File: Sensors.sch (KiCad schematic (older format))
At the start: 21 parts, among them U1 MCP60x4, U2 HTU21D, U3 PIR

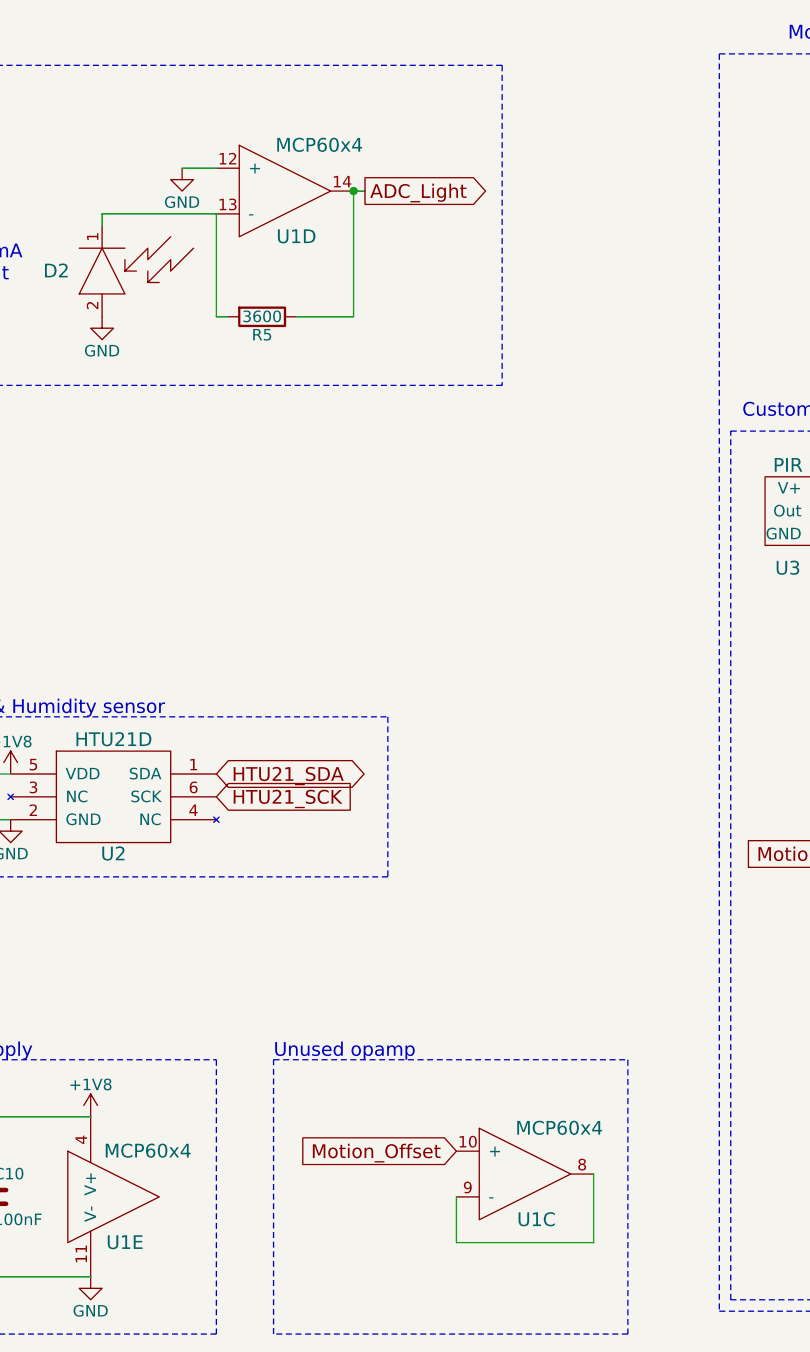
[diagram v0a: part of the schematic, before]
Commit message: Finish routing v4
Signed-off-by: pluyckx <philip.luyckx@gmail.com>
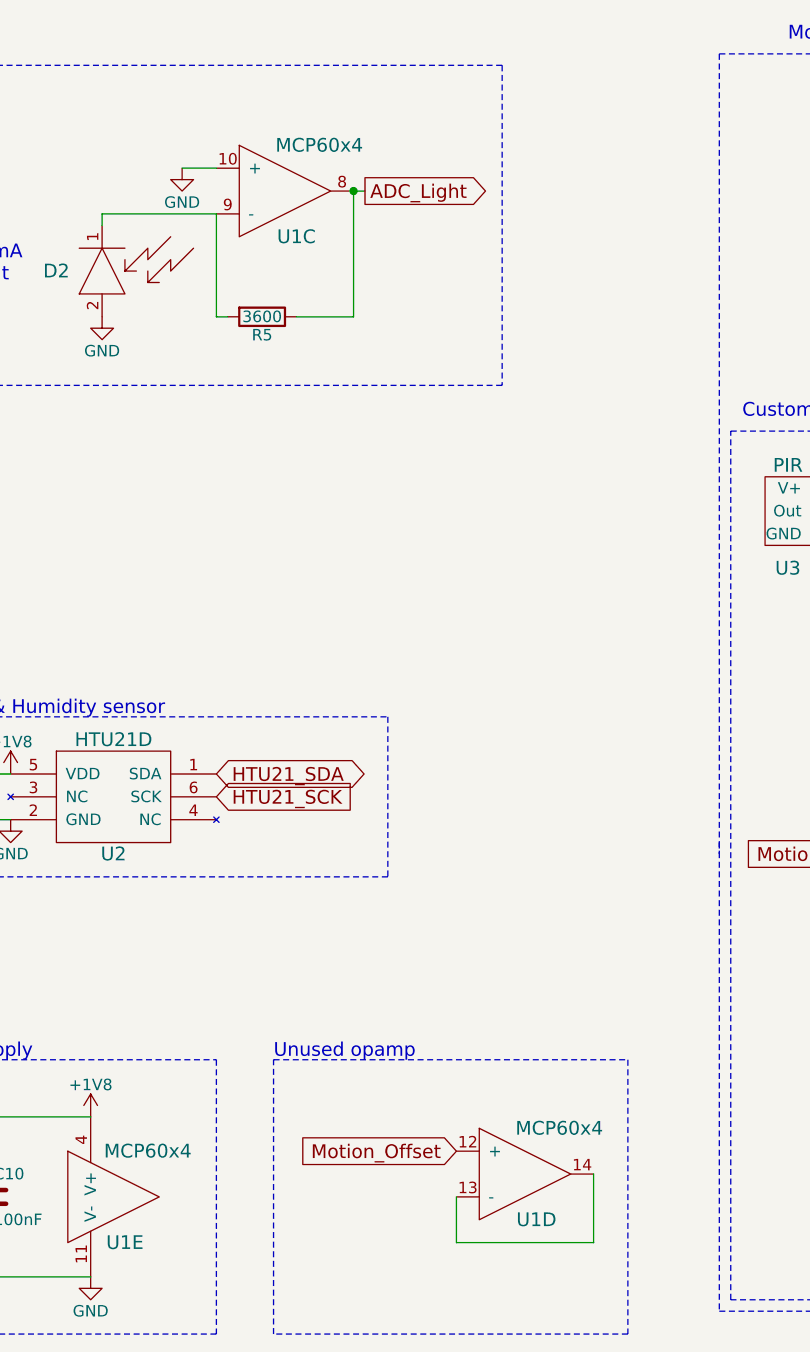
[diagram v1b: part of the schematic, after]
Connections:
- net ADC_Light: now also U1.8; no longer U1.14
- net GND: now also U1.10 (+); no longer U1.12 (+)
- net Motion_Offset: now also U1.12 (+); no longer U1.10 (+)
- net at D2.1, R5.2: now also U1.9 (-); no longer U1.13 (-)
- new net: U1.13 (-), U1.14
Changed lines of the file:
@@
 $Comp
 L MCP60x4 U1
-U 4 1 57538AEE
+U 3 1 57538AEE
 P 2650 1150
 F 0 "U1" H 2750 750 60  0000 C CNN
@@
 F 2 "CustomSmd:SOIC-14" H 2650 1150 60  0001 C CNN
 F 3 "" H 2650 1150 60  0000 C CNN
-	4    2650 1150
+	3    2650 1150
 	1    0    0    -1
 $EndComp
@@
 $Comp
 L MCP60x4 U1
-U 3 1 57538FA3
+U 4 1 57538FA3
 P 3700 5450
 F 0 "U1" H 3800 5050 60  0000 C CNN
@@
 F 2 "CustomSmd:SOIC-14" H 3700 5450 60  0001 C CNN
 F 3 "" H 3700 5450 60  0000 C CNN
-	3    3700 5450
+	4    3700 5450
 	1    0    0    -1
 $EndComp

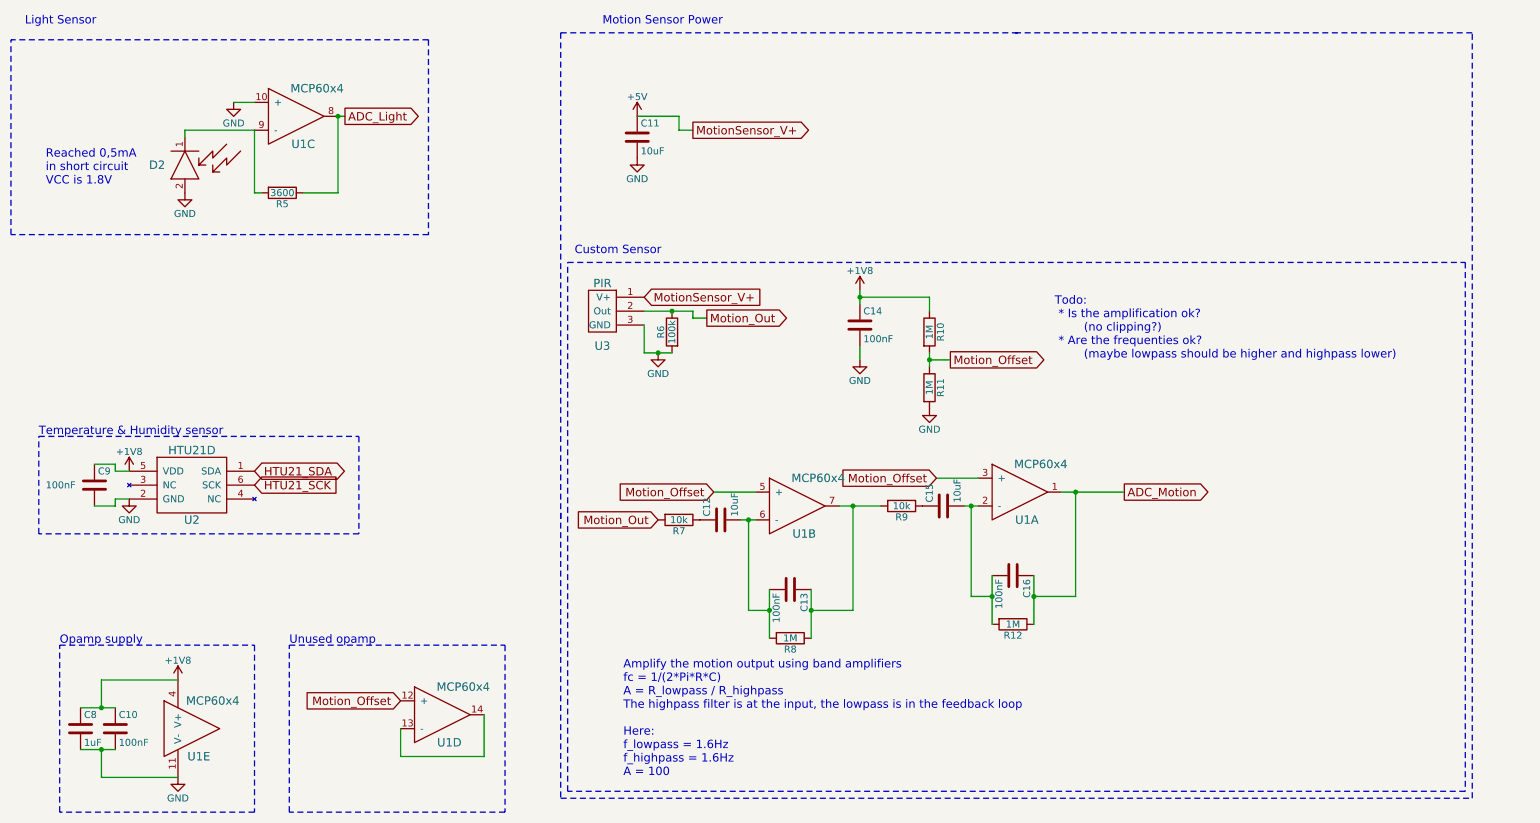
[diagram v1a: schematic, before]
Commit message: Update some routing
Signed-off-by: pluyckx <philip.luyckx@gmail.com>
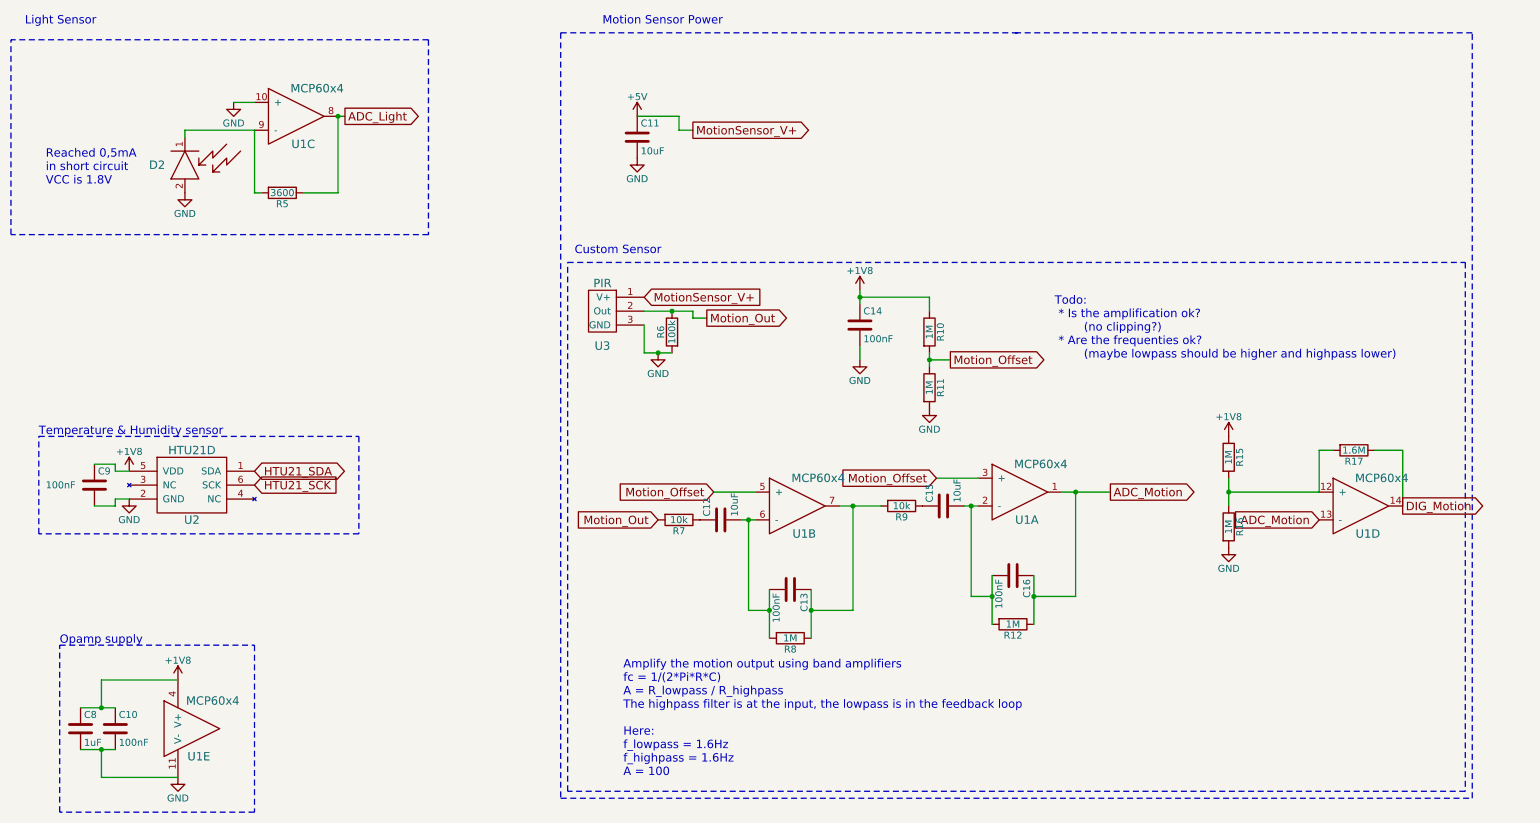
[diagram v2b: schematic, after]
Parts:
- added R15, R16: 1M, Resistors_SMD:R_0603, symbol R
- added R17: 1.6M, Resistors_SMD:R_0603, symbol R
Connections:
- net +1V8: now also R15.1
- net ADC_Motion: now also U1.13 (-)
- net GND: now also R16.2
- net Motion_Offset: no longer U1.12 (+)
- net DIG_Motion: now reaches U1.14
- net DIG_Motion: now also R17.1; no longer U1.13 (-)
- new net: R15.2, R16.1, R17.2, U1.12 (+)
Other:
- note removed: "Unused opamp"
- moved on the sheet: U1D
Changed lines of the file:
@@
 Wire Wire Line
 	8300 4800 8300 4050
-Wire Wire Line
-	8200 4050 8650 4050
 Connection ~ 8000 4800
 Wire Wire Line
@@
 Connection ~ 6700 4150
 Connection ~ 8300 4050
-Text GLabel 8650 4050 2    60   Output ~ 0
+Text GLabel 8550 4050 2    60   Output ~ 0
 ADC_Motion
 Text Notes 5050 6100 0    60   ~ 0
@@
 Text Notes 850  3650 0    60   ~ 0
 Temperature & Humidity sensor
-Wire Wire Line
-	3450 5750 3450 5950
-Wire Wire Line
-	3450 5950 4050 5950
 $Comp
 L MCP60x4 U1
@@
 L MCP60x4 U1
 U 4 1 57538FA3
-P 3700 5450
-F 0 "U1" H 3800 5050 60  0000 C CNN
-F 1 "MCP60x4" H 3900 5450 60  0000 C CNN
-F 2 "CustomSmd:SOIC-14" H 3700 5450 60  0001 C CNN
-F 3 "" H 3700 5450 60  0000 C CNN
-	4    3700 5450
+P 10300 3950
+F 0 "U1" H 10400 3550 60  0000 C CNN
+F 1 "MCP60x4" H 10500 3950 60  0000 C CNN
+F 2 "CustomSmd:SOIC-14" H 10300 3950 60  0001 C CNN
+F 3 "" H 10300 3950 60  0000 C CNN
+	4    10300 3950
 	1    0    0    -1
 $EndComp
@@
 Wire Wire Line
 	1300 5400 1850 5400
-Wire Wire Line
-	4050 5950 4050 5650
-Text GLabel 3450 5550 0    60   Input ~ 0
-Motion_Offset
 Wire Notes Line
 	1000 5150 2400 5150
@@
 Wire Notes Line
 	1000 6350 1000 5150
-Wire Notes Line
-	2650 5150 4200 5150
-Wire Notes Line
-	4200 5150 4200 6350
-Wire Notes Line
-	4200 6350 2650 6350
-Wire Notes Line
-	2650 6350 2650 5150
 Text Notes 1000 5150 0    60   ~ 0
 Opamp supply
-Text Notes 2650 5150 0    60   ~ 0
-Unused opamp
 Wire Wire Line
 	7250 2650 7250 2750
@@
 	1    0    0    -1
 $EndComp
+Text GLabel 10050 4250 0    60   Input ~ 0
+ADC_Motion
+$Comp
+L R R15
+U 1 1 57802832
+P 9400 3800
+F 0 "R15" V 9480 3800 50  0000 C CNN
+F 1 "1M" V 9400 3800 50  0000 C CNN
+F 2 "Resistors_SMD:R_0603" V 9330 3800 50  0001 C CNN
+F 3 "" H 9400 3800 50  0000 C CNN
+	1    9400 3800
+	1    0    0    -1
+$EndComp
+$Comp
+L R R16
+U 1 1 578028BF
+P 9400 4300
+F 0 "R16" V 9480 4300 50  0000 C CNN
+F 1 "1M" V 9400 4300 50  0000 C CNN
+F 2 "Resistors_SMD:R_0603" V 9330 4300 50  0001 C CNN
+F 3 "" H 9400 4300 50  0000 C CNN
+	1    9400 4300
+	1    0    0    -1
+$EndComp
+$Comp
+L +1V8 #PWR031
+U 1 1 5780291A
+P 9400 3650
+F 0 "#PWR031" H 9400 3500 50  0001 C CNN
+F 1 "+1V8" H 9400 3790 50  0000 C CNN
+F 2 "" H 9400 3650 50  0000 C CNN
+F 3 "" H 9400 3650 50  0000 C CNN
+	1    9400 3650
+	1    0    0    -1
+$EndComp
+Wire Wire Line
+	9400 3950 9400 4150
+$Comp
+L GND #PWR032
+U 1 1 578029DA
+P 9400 4450
+F 0 "#PWR032" H 9400 4200 50  0001 C CNN
+F 1 "GND" H 9400 4300 50  0000 C CNN
+F 2 "" H 9400 4450 50  0000 C CNN
+F 3 "" H 9400 4450 50  0000 C CNN
+	1    9400 4450
+	1    0    0    -1
+$EndComp
+Wire Wire Line
+	9400 4050 10050 4050
+Connection ~ 9400 4050
+Wire Wire Line
+	10050 4050 10050 3750
+Wire Wire Line
+	10050 3750 10150 3750
+$Comp
+L R R17
+U 1 1 57802B72
+P 10300 3750
+F 0 "R17" V 10380 3750 50  0000 C CNN
+F 1 "1.6M" V 10300 3750 50  0000 C CNN
+F 2 "Resistors_SMD:R_0603" V 10230 3750 50  0001 C CNN
+F 3 "" H 10300 3750 50  0000 C CNN
+	1    10300 3750
+	0    1    1    0
+$EndComp
+Wire Wire Line
+	10450 3750 10650 3750
+Wire Wire Line
+	10650 3750 10650 4150
+Text GLabel 10650 4150 2    60   Output ~ 0
+DIG_Motion
+Wire Wire Line
+	8200 4050 8550 4050
 $EndSCHEMATC
